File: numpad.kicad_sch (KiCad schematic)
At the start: 53 parts, among them SW2 SW_Push, U1 BlackPill_STLINK, U4 TRRS

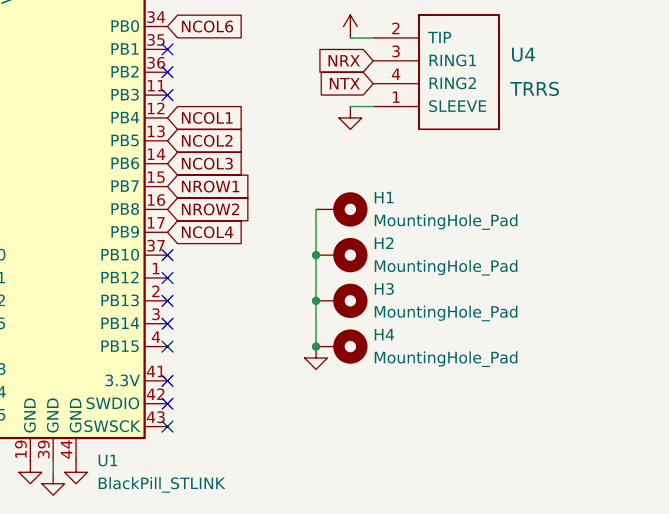
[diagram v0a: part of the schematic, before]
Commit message: Manufacturing Prep
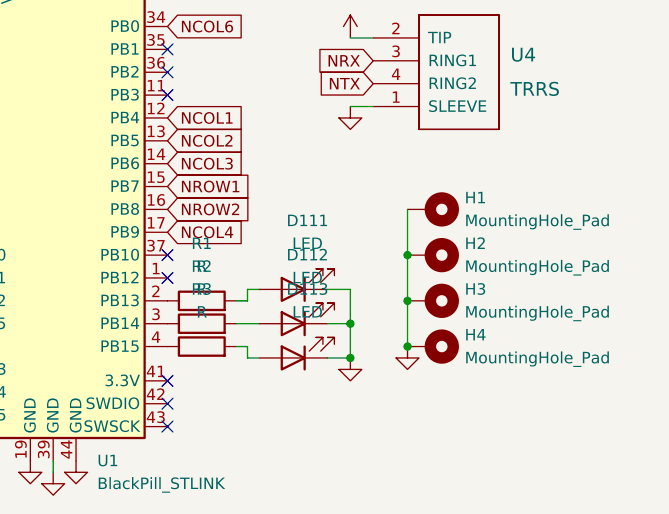
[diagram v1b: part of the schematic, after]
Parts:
- added D111, D112, D113: LED, LED_THT:LED_D5.0mm_Clear, symbol Device:LED
- added R1, R2, R3: R, Keebio-Parts:Resistor, symbol Device:R
- SW2: footprint Keebio-Parts:SW_Tactile_SPST_Angled_MJTP1117 -> Button_Switch_SMD:SW_SPST_PTS645Sx43SMTR92
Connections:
- net NGND: now also D111.1 (K), D112.1 (K), D113.1 (K)
- net at U1.2 (PB13): now also R1.1
- net at U1.3 (PB14): now also R2.1
- net at U1.4 (PB15): now also R3.1
- new net: D112.2 (A), R2.2
- new net: D113.2 (A), R3.2
- new net: D111.2 (A), R1.2
- no-connect marks 25 -> 22
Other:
- moved on the sheet: H1, H2, H3, H4
